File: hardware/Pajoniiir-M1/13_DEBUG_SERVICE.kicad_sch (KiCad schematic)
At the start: 15 parts

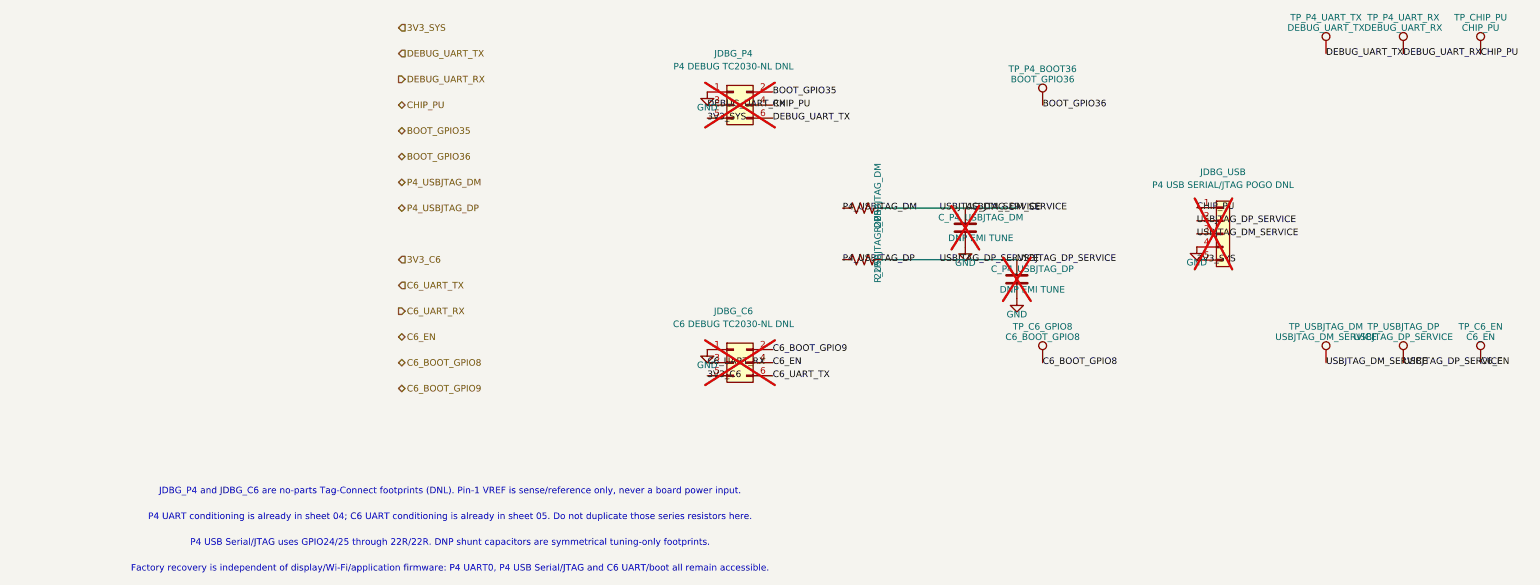
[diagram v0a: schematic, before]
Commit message: hardware: snap child sheets 11-15 to 25 mil grid
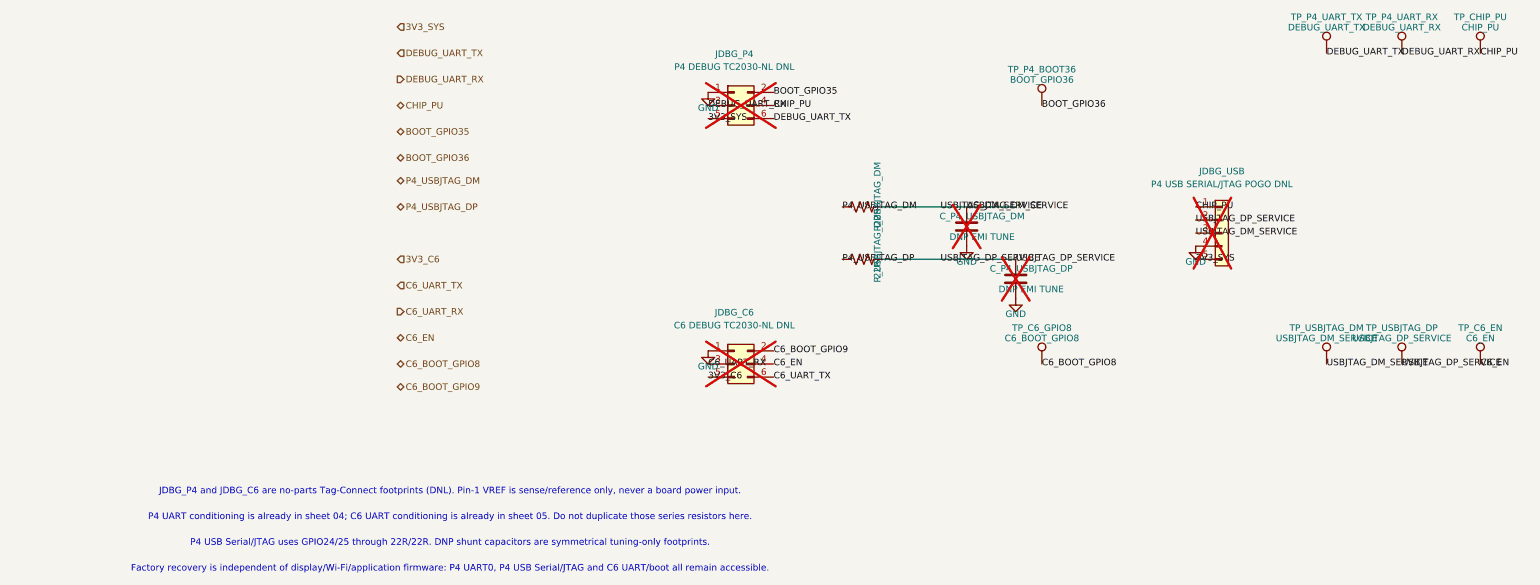
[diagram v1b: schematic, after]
